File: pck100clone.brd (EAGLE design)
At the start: 72.4 x 67 mm, 91 parts, among them IC1 LM358N, IC3 LM358N, IC4 LM358N, IC5 LM358N, Q1 2SC945, Q2 2SC945, Q3 2N3906, Q4 2N3906, Q5 2N3904, Q6 2N3904

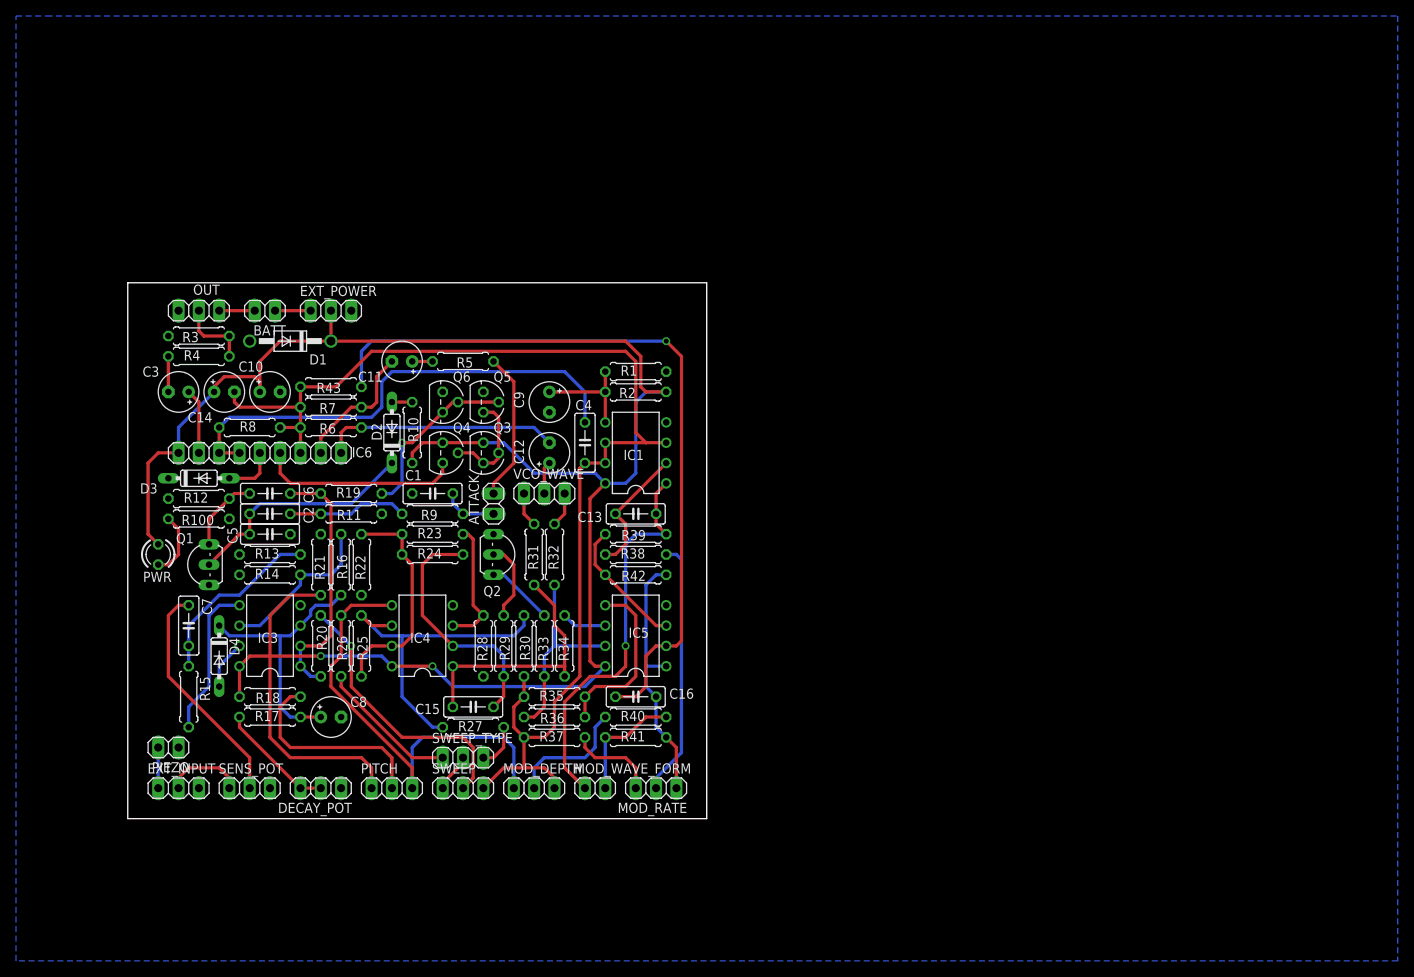
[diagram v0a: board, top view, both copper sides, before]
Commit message: almost done?
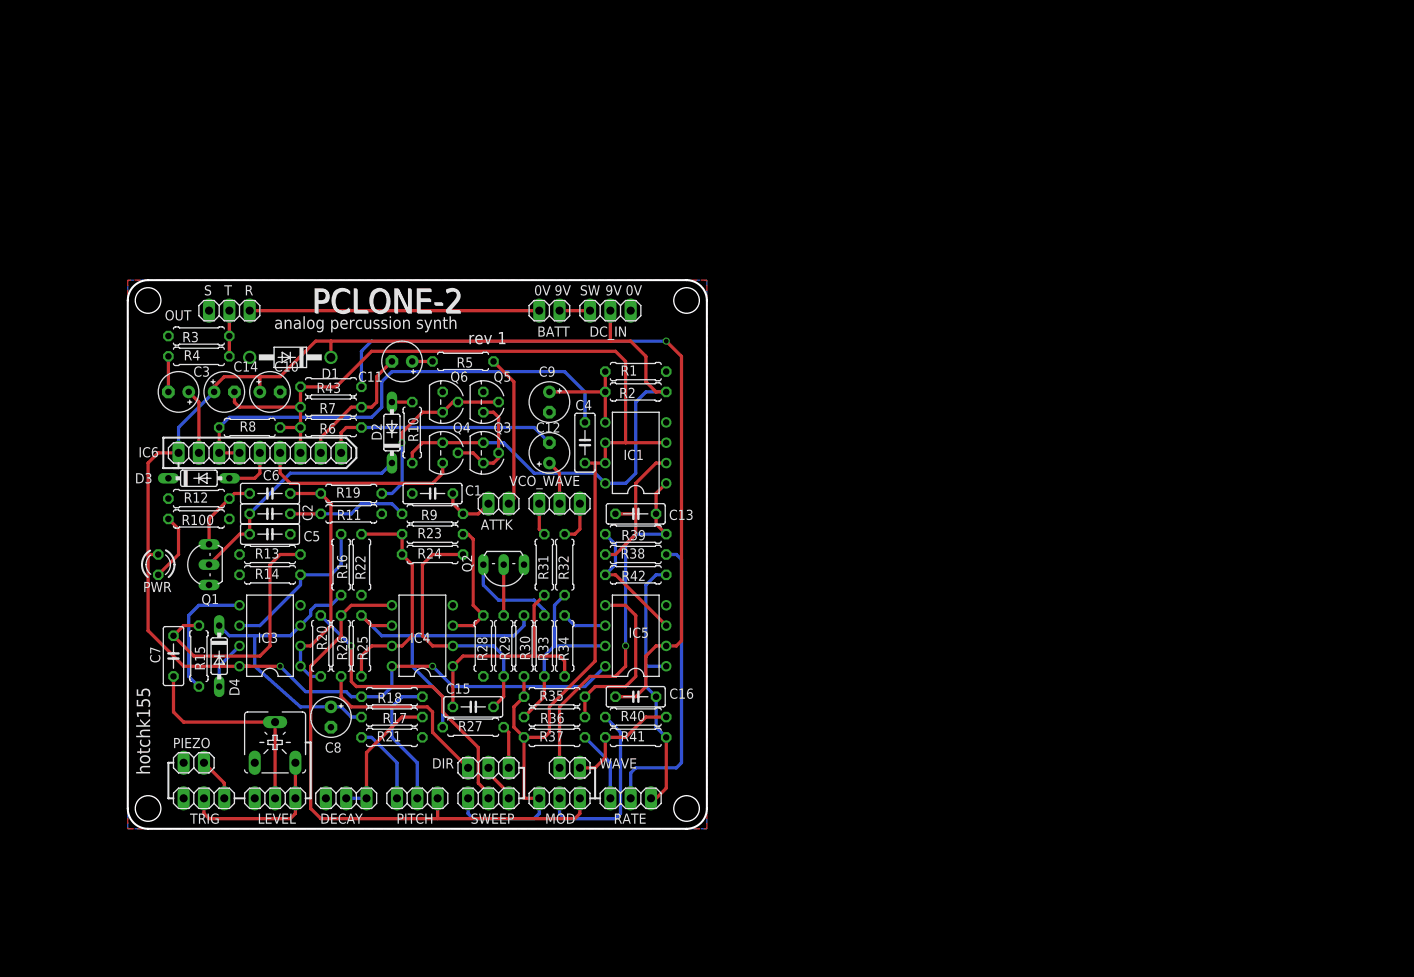
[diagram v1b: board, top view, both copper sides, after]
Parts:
- removed ATTACK, MOD_WAVE_FORM: (no value), pinhead:1X02
- removed DECAY_POT, EXT_INPUT, EXT_POWER, MOD_DEPTH, MOD_RATE, SENS_POT, SWEEP_TYPE: (no value), pinhead:1X03
- added ATTK, WAVE: (no value), pinhead:1X02
- added DC_IN, DECAY, DIR, LEVEL, MOD, RATE, TRIG: (no value), pinhead:1X03
- added SENS: (no value), pot:CA6V
- moved BATT 35.6 mm to (61.6, 66.0)
- moved R21 23.3 mm to (41.9, 12.7), turned to 0 degrees
- moved R17 15.2 mm to (41.9, 15.2), turned to 180 degrees
- moved R18 15.2 mm to (41.9, 17.8)
- moved R15 5.24 mm to (17.8, 22.9)
- moved C7 4.26 mm to (14.6, 22.9), turned to 90 degrees
- moved OUT 3.81 mm to (21.6, 66.0)
- moved PIEZO 3.70 mm to (17.1, 9.53), turned to 0 degrees
- moved PITCH 3.42 mm to (45.1, 5.08)
- moved SWEEP 3.42 mm to (54.0, 5.08), turned to 180 degrees
- moved VCO_WAVE 2.29 mm to (62.9, 41.9)
- moved D1 2.03 mm to (29.2, 60.2)
- moved Q2 1.80 mm to (55.9, 34.3), turned to 180 degrees
- moved R31 1.80 mm to (61.0, 34.3)
- moved R32 1.80 mm to (63.5, 34.3)
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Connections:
- net ATTACK_OUT: now also ATTK.2; no longer ATTACK.2
- net GND: now also DC_IN.3, DECAY.1, LEVEL.3, SENS.A, TRIG.3; no longer DECAY_POT.1, EXT_INPUT.3, EXT_POWER.3, SENS_POT.3
- net MOD_OUT: now also WAVE.2; no longer MOD_WAVE_FORM.2
- net N$1: now also TRIG.1; no longer EXT_INPUT.1
- net N$14: now also ATTK.1; no longer ATTACK.1
- net N$15: now also WAVE.1; no longer MOD_WAVE_FORM.1
- net N$17: now also RATE.2; no longer MOD_RATE.2
- net N$18: now also DIR.2; no longer SWEEP_TYPE.2
- net N$2: now also LEVEL.1, SENS.E, TRIG.2; no longer EXT_INPUT.2, SENS_POT.1
- net N$20: now also RATE.1; no longer MOD_RATE.1
- net N$22: now also RATE.3; no longer MOD_RATE.3
- net N$24: now also DIR.3; no longer SWEEP_TYPE.3
- net N$25: now also DIR.1; no longer SWEEP_TYPE.1
- net N$27: now also MOD.1; no longer MOD_DEPTH.1
- net N$28: now also MOD.2; no longer MOD_DEPTH.2
- net N$3: now also LEVEL.2, SENS.S; no longer SENS_POT.2
- net N$54: now also DC_IN.1; no longer EXT_POWER.1
- net N$9: now also DECAY.2, DECAY.3; no longer DECAY_POT.2, DECAY_POT.3
- net VCC: now also DC_IN.2; no longer EXT_POWER.2
- net VGND: now also MOD.3; no longer MOD_DEPTH.3
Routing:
- net N$50: track 4.45 -> 36.2 mm
- net N$30: track 39.5 -> 10.2 mm
- net N$27: track 57.1 -> 71.5 mm
- net N$2: track 9.94 -> 20.2 mm
- net N$4: track 22.7 -> 31.8 mm
- net N$29: track 25.7 -> 17.1 mm
- net N$28: track 15.5 -> 22.9 mm
- net VGND: track 151.4 -> 157.3 mm
- net N$25: track 17.7 -> 23.6 mm
- net N$17: track 32.1 -> 37.6 mm
- net N$8: track 32.7 -> 37.8 mm
- net N$36: track 8.45 -> 12.1 mm
- net N$35: track 9.94 -> 6.35 mm
- net OUT: track 9.15 -> 5.72 mm
- net N$15: track 49.6 -> 46.2 mm
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- added copper zone on layer 1, net GND
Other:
- board size 72.4 x 67 mm -> 72.4 x 68.6 mm
- board text added: "0V"
- board text added: "9V"
- board text added: "PCLONE-2"
- board text added: "R"
- board text added: "S"
- board text added: "SW"
- board text added: "T"
- board text added: "analog percussion synth"
- board text added: "hotchk155"
- board text added: "rev 1"
